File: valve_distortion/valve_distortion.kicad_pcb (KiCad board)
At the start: 2 copper layers, 116.8 x 31.8 mm, 30 parts, among them J1 INPUT, J2 OUTPUT, J3 Barrel_Jack, SW1 SW_DPDT_x2, U1 12AX7, U2 TL074

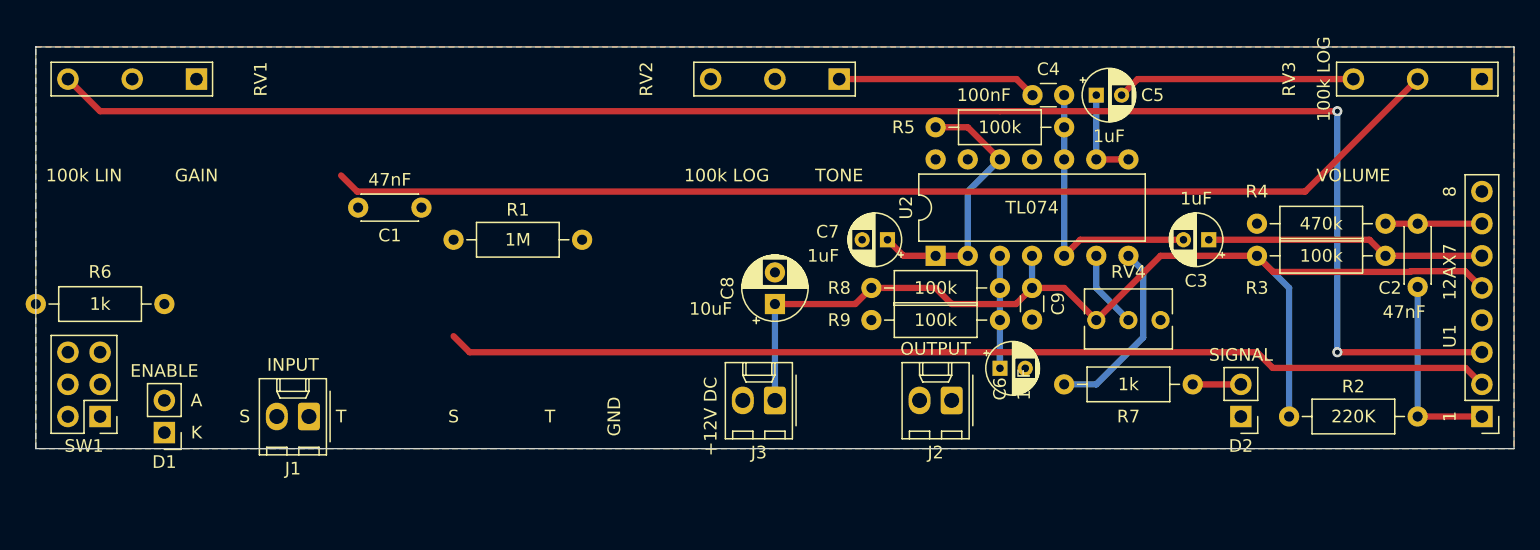
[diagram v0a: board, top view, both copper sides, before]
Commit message: Finish layout
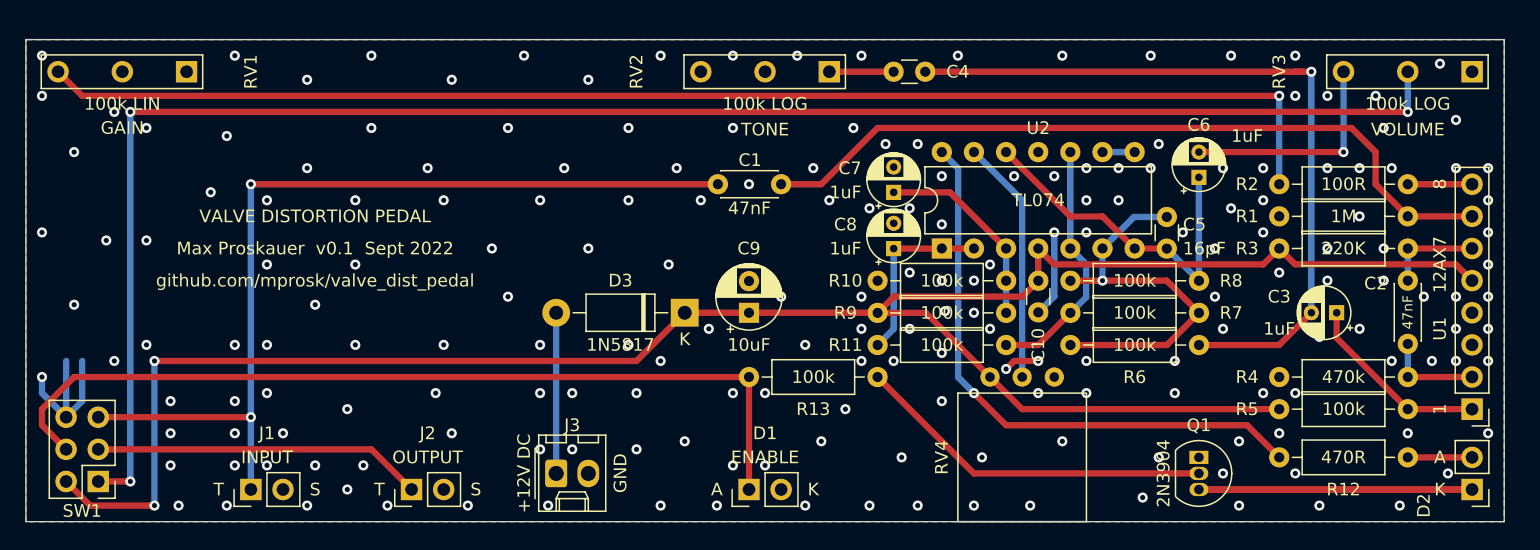
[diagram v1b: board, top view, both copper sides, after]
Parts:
- added C10: 0.1uF, Capacitor_THT:C_Disc_D3.0mm_W1.6mm_P2.50mm, F.Cu at (143.5, 82.6)
- added D3: 1N5817, Diode_THT:D_DO-41_SOD81_P10.16mm_Horizontal, F.Cu at (115.6, 85.1)
- added Q1: 2N3904, Package_TO_SOT_THT:TO-92_Inline, F.Cu at (156.2, 96.5)
- added R10: 100k, Resistor_THT:R_Axial_DIN0207_L6.3mm_D2.5mm_P10.16mm_Horizontal, F.Cu at (141.0, 82.6)
- added R11: 100k, Resistor_THT:R_Axial_DIN0207_L6.3mm_D2.5mm_P10.16mm_Horizontal, F.Cu at (141.0, 87.6)
- added R12: 470R, Resistor_THT:R_Axial_DIN0207_L6.3mm_D2.5mm_P10.16mm_Horizontal, F.Cu at (162.6, 96.5)
- added R13: 100k, Resistor_THT:R_Axial_DIN0207_L6.3mm_D2.5mm_P10.16mm_Horizontal, F.Cu at (130.8, 90.2)
- C5: value 1uF -> 16pF; footprint Capacitor_THT:CP_Radial_D4.0mm_P2.00mm -> Capacitor_THT:C_Disc_D3.0mm_W1.6mm_P2.50mm
- C8: value 10uF -> 1uF; footprint Capacitor_THT:CP_Radial_D5.0mm_P2.50mm -> Capacitor_THT:CP_Radial_D4.0mm_P2.00mm
- C9: value 0.1uF -> 10uF; footprint Capacitor_THT:C_Disc_D3.0mm_W1.6mm_P2.50mm -> Capacitor_THT:CP_Radial_D5.0mm_P2.50mm
- D1: value ENABLE -> LED IND 12V
- D2: value SIGNAL -> NTE30033
- J1, J2: footprint Connector_Molex:Molex_KK-254_AE-6410-02A_1x02_P2.54mm_Vertical -> Connector_PinHeader_2.54mm:PinHeader_1x02_P2.54mm_Vertical
- R2: value 220K -> 100R
- R3: value 100k -> 220K
- R6, R7: value 1k -> 100k
- RV4: value R_Potentiometer_Trim -> 200k; footprint Potentiometer_THT:Potentiometer_Bourns_3266Y_Vertical -> valve_distortion:Trimmer
- moved R1 75.4 mm to (172.7, 77.5), turned to 180 degrees
- moved R6 71.7 mm to (146.1, 87.6), turned to 0 degrees
- moved D1 46.4 mm to (120.7, 99.1), turned to 90 degrees
- moved J2 43.3 mm to (94.0, 99.1), turned to 90 degrees
- moved C1 28.5 mm to (123.2, 74.9)
- moved R5 28.0 mm to (162.6, 92.7), turned to 0 degrees
- moved R8 25.9 mm to (156.2, 82.6), turned to 180 degrees
- moved C9 22.5 mm to (120.7, 85.1), turned to 90 degrees
- moved C6 21.8 mm to (156.2, 74.4), turned to 90 degrees
- moved R2 20.6 mm to (172.7, 74.9), turned to 180 degrees
- moved D2 19.2 mm to (177.8, 99.1)
- moved J3 18.2 mm to (105.4, 97.8), turned to 0 degrees
- moved C5 13.3 mm to (153.7, 80.0), turned to 90 degrees
- moved R4 12.2 mm to (172.7, 90.2)
- moved R7 12.1 mm to (156.2, 85.1), turned to 180 degrees
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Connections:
- C5 pad 1: Net-(C5-Pad1) -> /BUF_OUT
- C5 pad 2: Net-(C5-Pad2) -> Net-(R6-Pad1)
- C6 pad 1: Net-(R8-Pad2) -> /BUF_OUT
- C6 pad 2: GND -> Net-(C6-Pad2)
- C7 pad 1: /VBIAS -> Net-(C7-Pad1)
- C8 pad 1: +12V -> Net-(C8-Pad1)
- D1 pad 1: GND -> /ENABLE
- D1 pad 2: Net-(D1-Pad2) -> GND
- D2 pad 1: GND -> Net-(D2-Pad1)
- D2 pad 2: Net-(R7-Pad2) -> Net-(D2-Pad2)
- J3 pad 1: +12V -> Net-(J3-Pad1)
- R2 pad 1: +12V -> Net-(R2-Pad1)
- R2 pad 2: Net-(C2-Pad2) -> Net-(R2-Pad2)
- R3 pad 2: Net-(C3-Pad1) -> Net-(C2-Pad2)
- R5 pad 1: Net-(C3-Pad2) -> +12V
- R5 pad 2: /VBIAS -> Net-(C3-Pad1)
- R6 pad 1: Net-(D1-Pad2) -> Net-(R6-Pad1)
- R6 pad 2: Net-(R6-Pad2) -> Net-(C3-Pad2)
- R7 pad 1: Net-(U2-Pad7) -> Net-(R6-Pad1)
- R7 pad 2: Net-(R7-Pad2) -> VBIAS
- R8 pad 1: +12V -> /BUF_OUT
- R8 pad 2: Net-(R8-Pad2) -> Net-(R6-Pad1)
- R9 pad 1: Net-(R8-Pad2) -> +12V
- R9 pad 2: GND -> Net-(C7-Pad1)
- RV1 pad 3: Net-(RV1-Pad3) -> Net-(R2-Pad2)
- RV3 pad 3: Net-(C5-Pad2) -> Net-(C6-Pad2)
- RV4 pad 2: Net-(RV4-Pad2) -> Net-(U2-Pad13)
- SW1 pad 4: Net-(R6-Pad2) -> +12V
- SW1 pad 5: +12V -> /ENABLE
- SW1 pad 6: unconnected-(SW1-Pad6) -> GND
- U1 pad 1: Net-(C2-Pad2) -> Net-(C3-Pad1)
- U1 pad 2: Net-(C1-Pad1) -> Net-(C2-Pad1)
- U1 pad 3: Net-(RV1-Pad3) -> GND
- U1 pad 6: Net-(C3-Pad1) -> Net-(C2-Pad2)
- U1 pad 7: Net-(C2-Pad1) -> Net-(C1-Pad1)
- U1 pad 8: GND -> Net-(R2-Pad1)
- U2 pad 1: /VBIAS -> Net-(C8-Pad1)
- U2 pad 10: Net-(C3-Pad2) -> VBIAS
- U2 pad 12: /VBIAS -> /BUF_OUT
- U2 pad 14: Net-(U2-Pad13) -> Net-(R12-Pad1)
- U2 pad 2: /VBIAS -> Net-(C8-Pad1)
- U2 pad 3: Net-(R8-Pad2) -> Net-(C7-Pad1)
- U2 pad 5: Net-(C3-Pad2) -> VBIAS
- U2 pad 6: Net-(RV4-Pad2) -> Net-(R6-Pad1)
- U2 pad 7: Net-(U2-Pad7) -> /BUF_OUT
- U2 pad 8: Net-(C5-Pad1) -> Net-(U2-Pad8)
- U2 pad 9: Net-(C5-Pad1) -> Net-(U2-Pad8)
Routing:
- net Net-(RV1-Pad3): track 131.9 -> 0.00 mm, vias 2 -> 0
- net Net-(R2-Pad2): track 0.00 -> 104.3 mm, vias 0 -> 1
- net +12V: track 85.6 -> 165.5 mm, vias 0 -> 2
- net /INPUT: track 0.00 -> 73.1 mm, vias 0 -> 2
- net /ENABLE: track 0.00 -> 69.8 mm
- net Net-(RV3-Pad2): track 89.3 -> 135.9 mm, vias 0 -> 3
- net Net-(R12-Pad1): track 0.00 -> 46.3 mm, vias 0 -> 1
- net Net-(C3-Pad2): track 22.7 -> 60.1 mm, vias 0 -> 1
- net Net-(R6-Pad1): track 0.00 -> 31.1 mm, vias 0 -> 1
- net Net-(Q1-Pad2): track 0.00 -> 28.6 mm
- net /BUF_OUT: track 0.00 -> 27.6 mm
- net Net-(J2-PadT): track 0.00 -> 26.1 mm
- net GND: track 0.00 -> 23.0 mm, vias 0 -> 200
- net Net-(C1-Pad1): track 82.9 -> 60.8 mm
- net /VBIAS: track 21.7 -> 0.00 mm
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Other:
- board size 116.8 x 31.8 mm -> 116.8 x 38.1 mm
- board text added: "ENABLE"
- board text added: "JLCJLCJLCJLC"
- board text added: "Max Proskauer v0.1 Sept 2022"
- board text added: "VALVE DISTORTION PEDAL"
- board text added: "github.com/mprosk/valve_dist_pedal"
